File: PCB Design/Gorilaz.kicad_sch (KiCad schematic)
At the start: 47 parts, among them J1 Conn_01x13, J2 Conn_01x13, J3 Conn_01x13, J4 Conn_01x13, J5 HRO_TYPE-C-31-M-14, J6 Battery, J7 Conn_01x13, J8 Conn_01x13, J9 TC2030_SWD, Q2 2N7002, SW1 PWR, SW4 RST, U1 SRV05-4, U10 MAX17048, U3 BQ24075, U4 DW01A, U5 FS8205, U8 nRF52840_moko_mk08

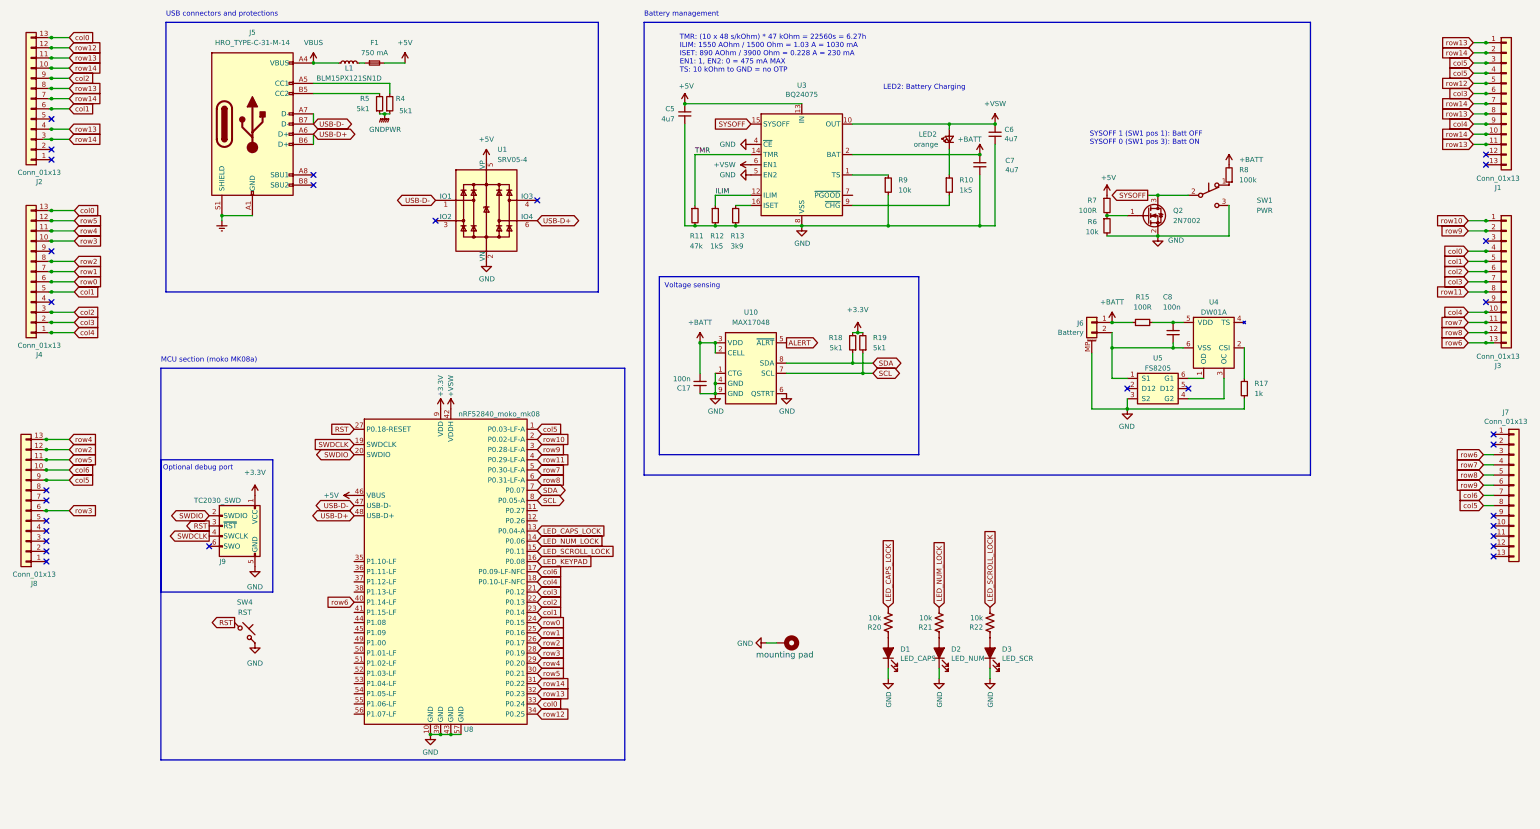
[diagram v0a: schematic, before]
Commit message: power managemnt rework
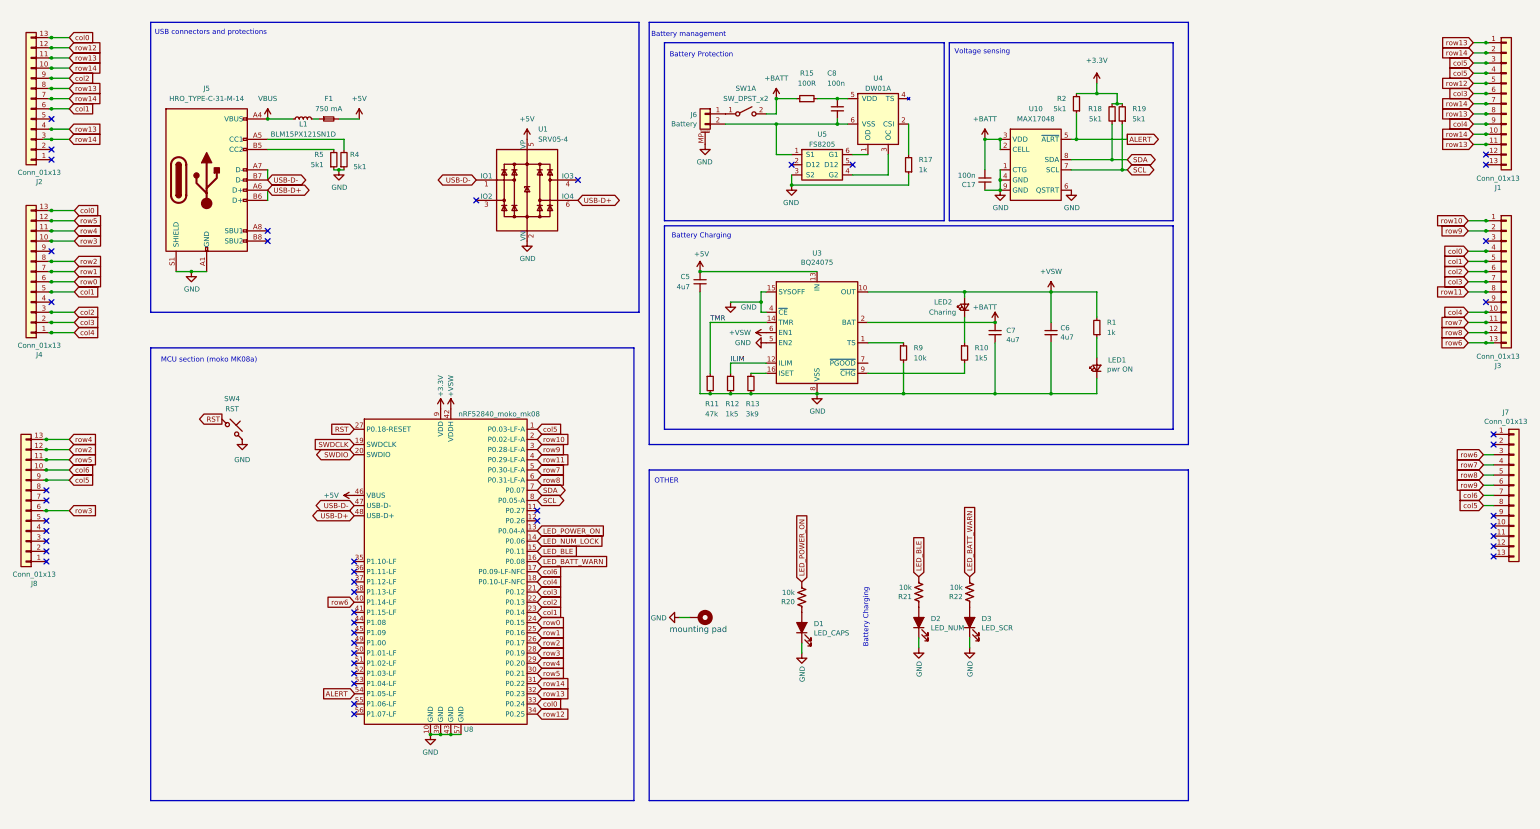
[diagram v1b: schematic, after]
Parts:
- removed J9: TC2030_SWD, Local:CON_TC2030_outlined, symbol PCM_marbastlib-various:TC2030_SWD
- removed Q2: 2N7002, Package_TO_SOT_SMD:SOT-23, symbol Transistor_FET:2N7002
- removed R6: 10k, Resistor_SMD:R_0402_1005Metric, symbol Device:R_Small
- removed R7: 100R, Resistor_SMD:R_0402_1005Metric, symbol Device:R_Small
- removed R8: 100k, Resistor_SMD:R_0402_1005Metric, symbol Device:R_Small
- removed SW1: PWR, Mastarlib:SW_MSK12C02-HB, symbol Switch:SW_Push_SPDT
- added LED1: pwr ON, LED_SMD:LED_0402_1005Metric, symbol Device:LED_Small
- added R1: 1k, Resistor_SMD:R_0402_1005Metric, symbol Device:R_Small
- added R2: 5k1, Resistor_SMD:R_0402_1005Metric, symbol Device:R_Small
- added SW1: SW_DPST_x2, symbol Switch:SW_DPST_x2
- LED2: value orange -> Charing
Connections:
- net GNDPWR is gone; now on net GND: R4.1, R5.1
- net SYSOFF is gone; now on net GND: U3.15 (SYSOFF)
- net +3.3V: now also R2.2
- net +BATT: now also SW1.2 (B); no longer J6.1 (Pin_1)
- net +VSW: now also R1.2
- net ALERT: now also R2.1
- net GND: now also LED1.1 (K)
- net LED_NUM_LOCK: no longer R21.2
- net LED_CAPS_LOCK renamed LED_POWER_ON
- net LED_KEYPAD renamed LED_BATT_WARN
- net LED_BATT_WARN: now also R22.2
- net LED_SCROLL_LOCK renamed LED_BLE
- net LED_BLE: now also R21.2; no longer R22.2
- new net: LED1.2 (A), R1.1
- new net: J6.1 (Pin_1), SW1.1 (A)
- no-connect marks 30 -> 45
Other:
- note added: "Battery Charging"
- note added: "Battery Protection"
- note added: "OTHER"
- note removed: "LED2: Battery Charging"
- note removed: "Optional debug port"
- note removed: "SYSOFF 1 (SW1 pos 1): Batt OFF SYSOFF 0 (SW1 pos 3): Batt ON"
- note removed: "TMR: (10 x 48 s/kOhm) * 47 kOhm = 22560s = 6.27h ILIM: 1550 AOhm / 1500 Ohm = 1.03 A = 1030 mA ISET: 890 AOhm / 3900 Ohm = 0.228 A = 230 mA EN1: 1, EN2: 0 = 475 mA MAX TS: 10 kOhm to GND = no OTP"
- moved on the sheet: C17, C5, C6, C7, C8, D1, D2, D3, F1, J5, J6, L1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

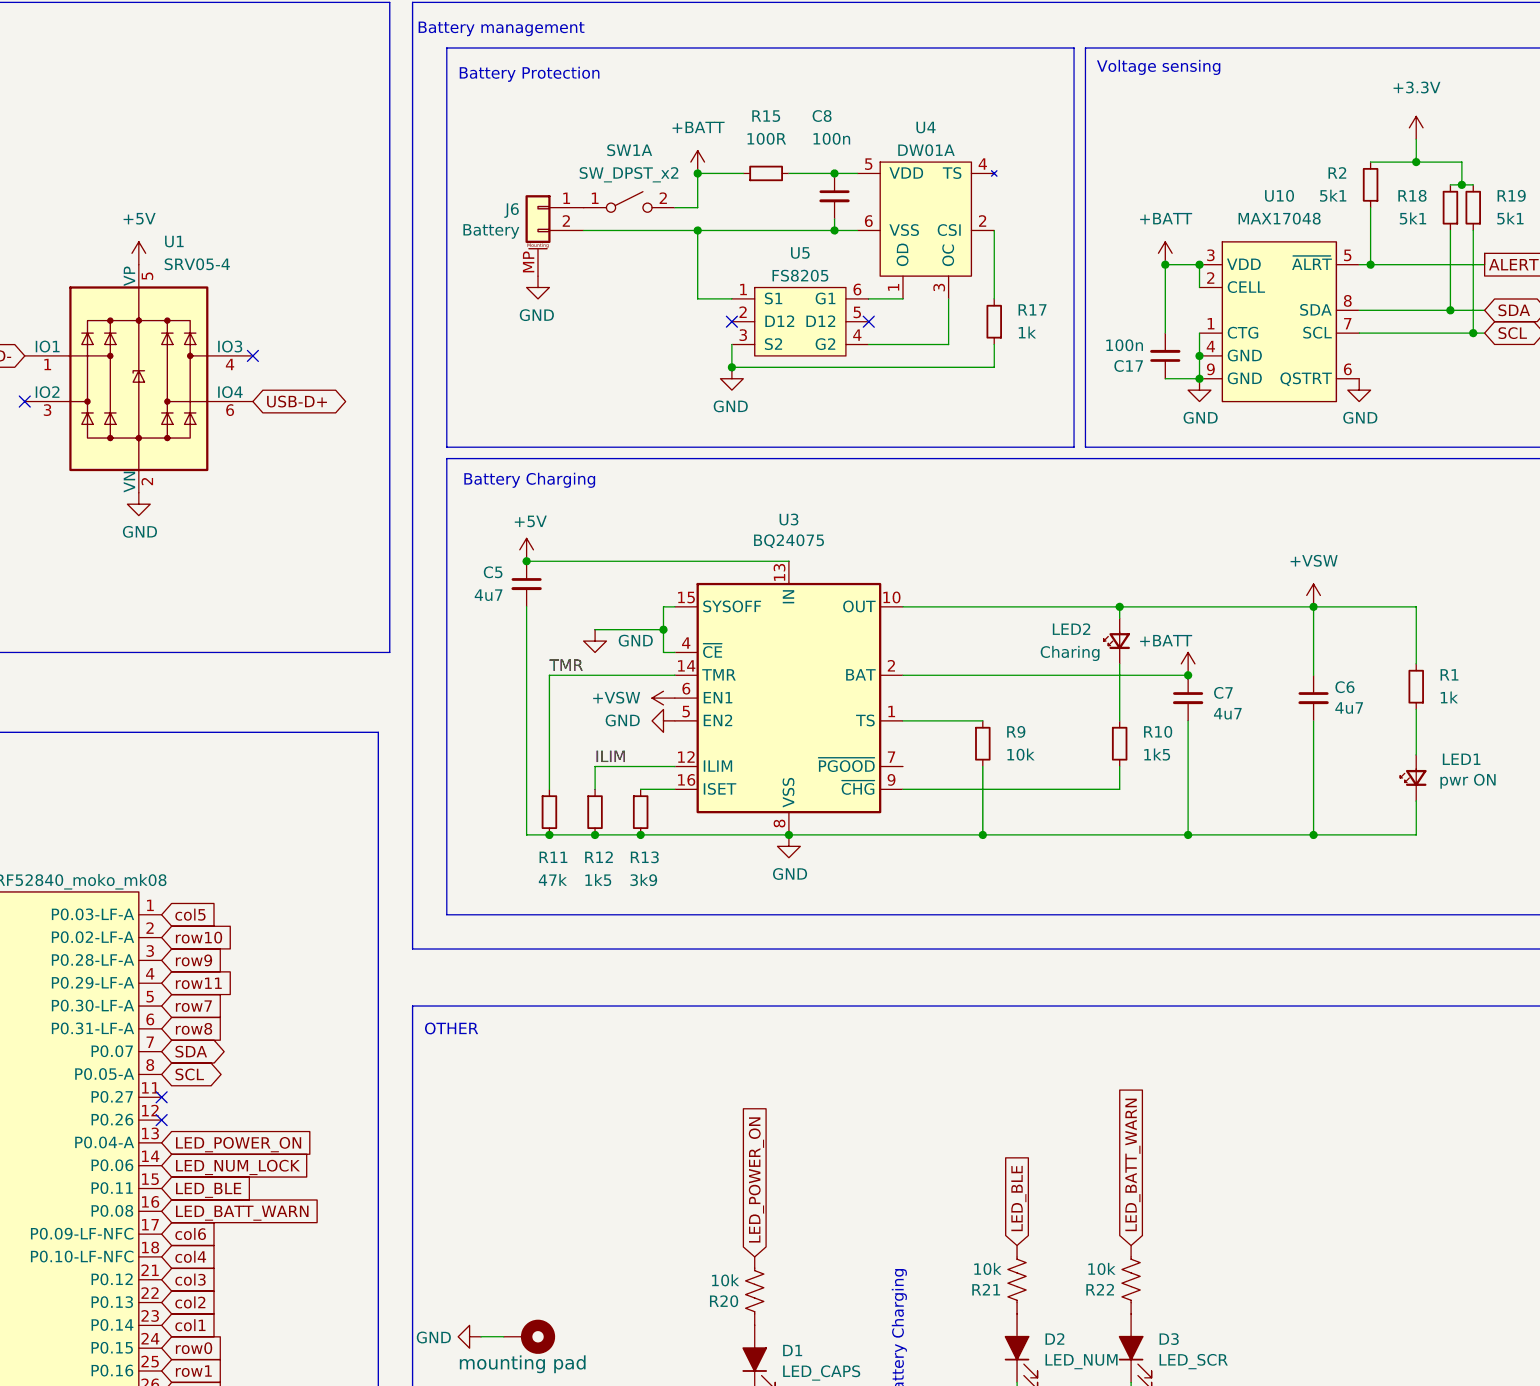
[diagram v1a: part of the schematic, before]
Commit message: big updates push
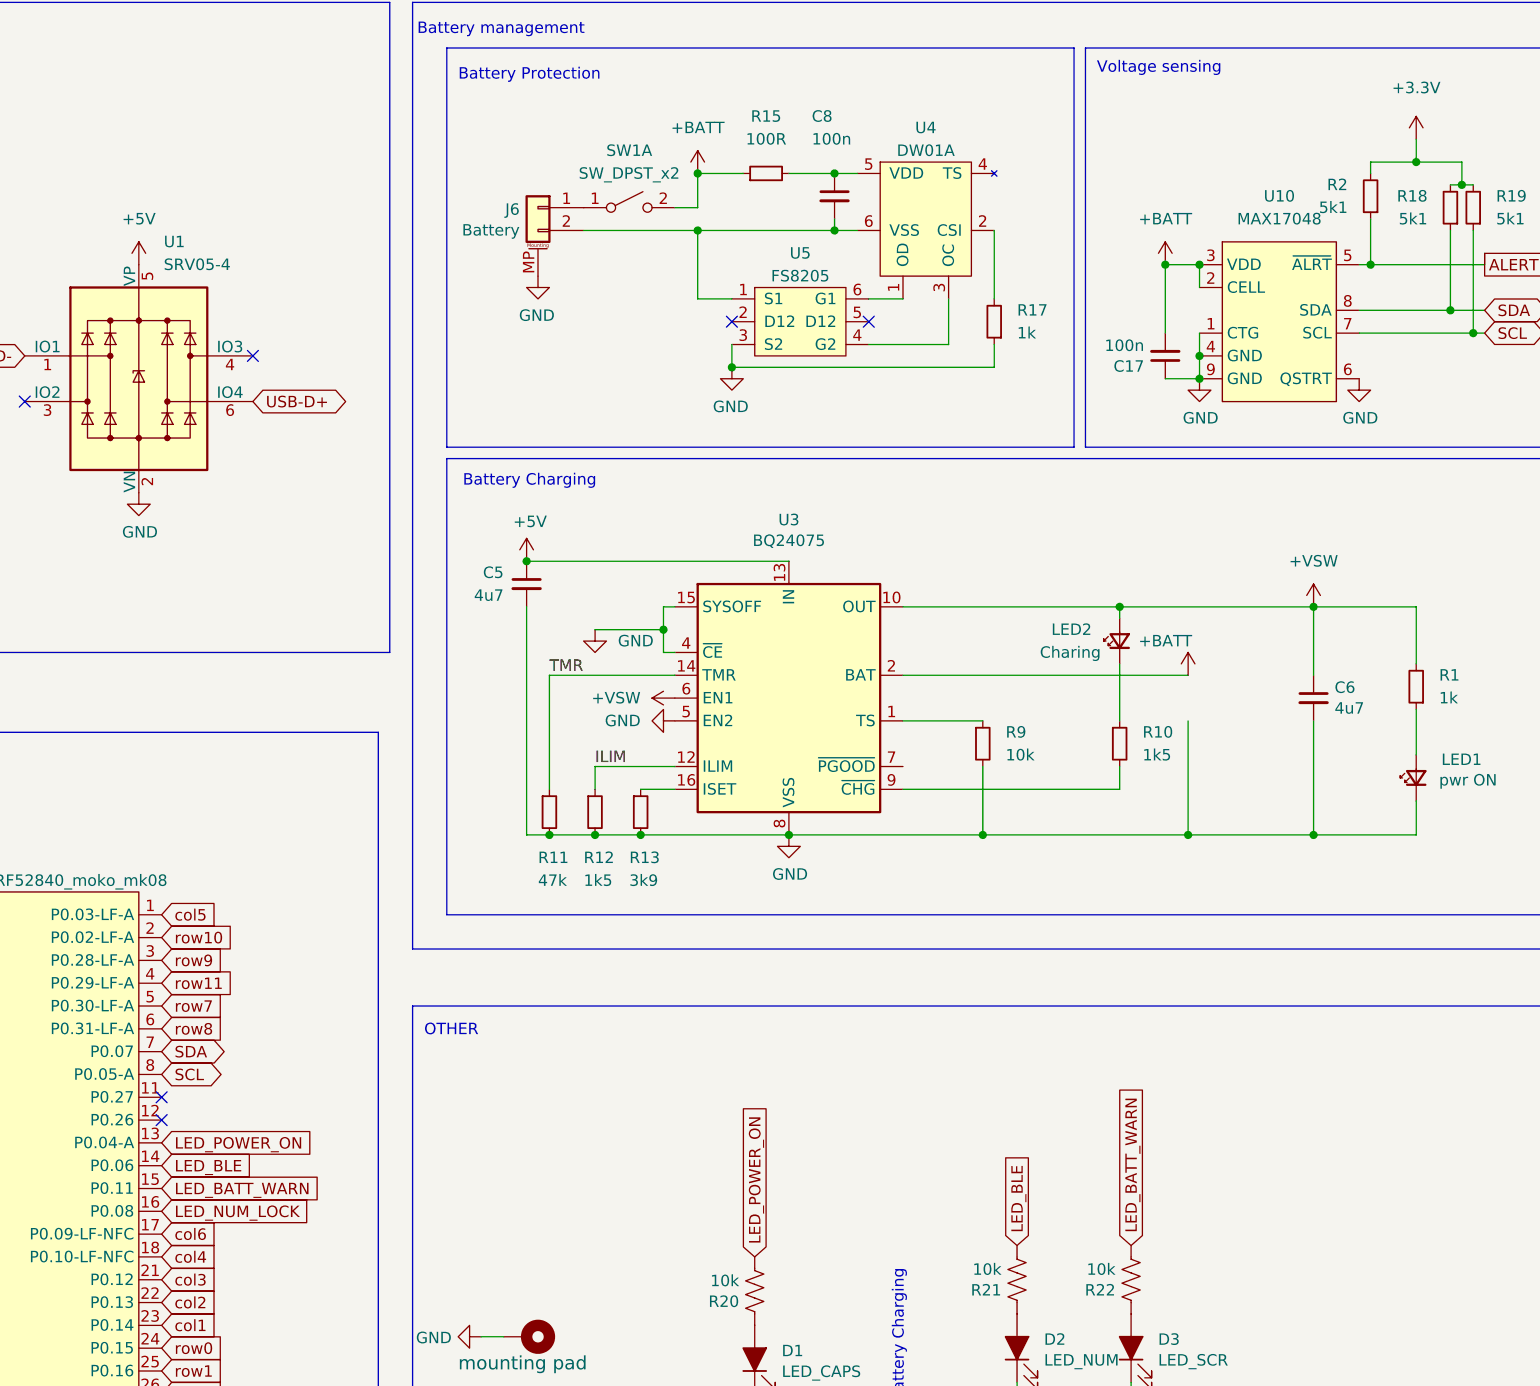
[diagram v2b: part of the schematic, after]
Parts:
- removed C7: 4u7, Capacitor_SMD:C_0402_1005Metric, symbol Device:C_Small
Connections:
- net LED_BATT_WARN: now also U8.15 (P0.11); no longer U8.16 (P0.08)
- net LED_BLE: now also U8.14 (P0.06); no longer U8.15 (P0.11)
- net LED_NUM_LOCK: now also U8.16 (P0.08); no longer U8.14 (P0.06)
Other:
- moved on the sheet: R2
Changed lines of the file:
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@@
 	)
 	(junction
-		(at 267.97 99.06)
-		(diameter 0.9144)
-		(color 0 0 0 0)
-	)
-	(junction
 		(at 132.08 201.93)
 		(diameter 0)
@@
 	(wire
 		(pts
-			(xy 293.37 41.91) (xy 298.45 41.91)
-		)
-		(stroke
-			(width 0)
-			(type default)
-		)
-	)
-	(wire
-		(pts
 			(xy 30.48 146.05) (xy 31.115 146.05)
 		)
@@
 	(wire
 		(pts
-			(xy 288.29 41.91) (xy 293.37 41.91)
-		)
-		(stroke
-			(width 0)
-			(type default)
-		)
-	)
-	(wire
-		(pts
 			(xy 390.525 39.37) (xy 391.16 39.37)
 		)
@@
 	(wire
 		(pts
+			(xy 293.37 41.91) (xy 298.45 41.91)
+		)
+		(stroke
+			(width 0)
+			(type default)
+		)
+	)
+	(wire
+		(pts
 			(xy 86.36 55.88) (xy 102.87 55.88)
 		)
@@
 	(wire
 		(pts
+			(xy 288.29 41.91) (xy 288.29 43.18)
+		)
+		(stroke
+			(width 0)
+			(type default)
+		)
+	)
+	(wire
+		(pts
 			(xy 31.75 50.8) (xy 32.385 50.8)
 		)
@@
 	(wire
 		(pts
-			(xy 288.29 46.99) (xy 288.29 53.34)
+			(xy 288.29 48.26) (xy 288.29 53.34)
 		)
 		(stroke
@@
 	(wire
 		(pts
+			(xy 288.29 41.91) (xy 293.37 41.91)
+		)
+		(stroke
+			(width 0)
+			(type default)
+		)
+	)
+	(wire
+		(pts
 			(xy 32.385 45.72) (xy 36.83 45.72)
 		)
@@
 		)
 	)
+	(global_label "LED_BATT_WARN"
+		(shape input)
+		(at 153.67 156.21 0)
+		(fields_autoplaced yes)
+		(effects
+			(font
+				(size 1.27 1.27)
+			)
+			(justify left)
+		)
+		(property "Intersheetrefs" "${INTERSHEET_REFS}"
+			(at 171.4718 156.21 0)
+			(effects
+				(font
+					(size 1.27 1.27)
+				)
+				(justify left)
+				(hide yes)
+			)
+		)
+	)
 	(global_label "col6"
 		(shape input)
@@
 		)
 	)
+	(global_label "LED_BLE"
+		(shape input)
+		(at 153.67 153.67 0)
+		(fields_autoplaced yes)
+		(effects
+			(font
+				(size 1.27 1.27)
+			)
+			(justify left)
+		)
+		(property "Intersheetrefs" "${INTERSHEET_REFS}"
+			(at 164.517 153.67 0)
+			(effects
+				(font
+					(size 1.27 1.27)
+				)
+				(justify left)
+				(hide yes)
+			)
+		)
+	)
 	(global_label "LED_BATT_WARN"
 		(shape input)
@@
 		)
 	)
-	(global_label "LED_BATT_WARN"
-		(shape input)
-		(at 153.67 158.75 0)
-		(fields_autoplaced yes)
-		(effects
-			(font
-				(size 1.27 1.27)
-			)
-			(justify left)
-		)
-		(property "Intersheetrefs" "${INTERSHEET_REFS}"
-			(at 171.4718 158.75 0)
-			(effects
-				(font
-					(size 1.27 1.27)
-				)
-				(justify left)
-				(hide yes)
-			)
-		)
-	)
 	(global_label "row4"
 		(shape input)
@@
 		)
 	)
-	(global_label "LED_BLE"
-		(shape input)
-		(at 153.67 156.21 0)
-		(fields_autoplaced yes)
-		(effects
-			(font
-				(size 1.27 1.27)
-			)
-			(justify left)
-		)
-		(property "Intersheetrefs" "${INTERSHEET_REFS}"
-			(at 164.517 156.21 0)
-			(effects
-				(font
-					(size 1.27 1.27)
-				)
-				(justify left)
-				(hide yes)
-			)
-		)
-	)
 	(global_label "col0"
 		(shape input)
@@
 		)
 	)
-	(global_label "LED_NUM_LOCK"
-		(shape input)
-		(at 153.67 153.67 0)
-		(fields_autoplaced yes)
-		(effects
-			(font
-				(size 1.27 1.27)
-			)
-			(justify left)
-		)
-		(property "Intersheetrefs" "${INTERSHEET_REFS}"
-			(at 171.0485 153.67 0)
-			(effects
-				(font
-					(size 1.27 1.27)
-				)
-				(justify left)
-				(hide yes)
-			)
-		)
-	)
 	(global_label "col6"
 		(shape input)
@@
 		)
 	)
+	(global_label "LED_NUM_LOCK"
+		(shape input)
+		(at 153.67 158.75 0)
+		(fields_autoplaced yes)
+		(effects
+			(font
+				(size 1.27 1.27)
+			)
+			(justify left)
+		)
+		(property "Intersheetrefs" "${INTERSHEET_REFS}"
+			(at 171.0485 158.75 0)
+			(effects
+				(font
+					(size 1.27 1.27)
+				)
+				(justify left)
+				(hide yes)
+			)
+		)
+	)
 	(global_label "LED_POWER_ON"
 		(shape input)
@@
 	)
 	(symbol
-		(lib_id "Device:C_Small")
-		(at 267.97 101.6 0)
-		(unit 1)
-		(exclude_from_sim no)
-		(in_bom yes)
-		(on_board yes)
-		(dnp no)
-		(property "Reference" "C7"
-			(at 270.764 101.0666 0)
-			(effects
-				(font
-					(size 1.27 1.27)
-				)
-				(justify left)
-			)
-		)
-		(property "Value" "4u7"
-			(at 270.764 103.378 0)
-			(effects
-				(font
-					(size 1.27 1.27)
-				)
-				(justify left)
-			)
-		)
-		(property "Footprint" "Capacitor_SMD:C_0402_1005Metric"
-			(at 267.97 101.6 0)
-			(effects
-				(font
-					(size 1.27 1.27)
-				)
-				(hide yes)
-			)
-		)
-		(property "Datasheet" "~"
-			(at 267.97 101.6 0)
-			(effects
-				(font
-					(size 1.27 1.27)
-				)
-				(hide yes)
-			)
-		)
-		(property "Description" ""
-			(at 267.97 101.6 0)
-			(effects
-				(font
-					(size 1.27 1.27)
-				)
-				(hide yes)
-			)
-		)
-		(property "LCSC" ""
-			(at 267.97 101.6 0)
-			(effects
-				(font
-					(size 1.27 1.27)
-				)
-				(hide yes)
-			)
-		)
-		(property "Notes" "X7R, 10%"
-			(at 267.97 101.6 0)
-			(effects
-				(font
-					(size 1.27 1.27)
-				)
-				(hide yes)
-			)
-		)
-		(pin "1"
-		)
-		(pin "2"
-		)
-		(instances
-			(project "Gorilaz"
-				(path "/46ef0abf-42df-44ff-8272-0b82956755c4"
-					(reference "C7")
-					(unit 1)
-				)
-			)
-		)
-	)
-	(symbol
 		(lib_id "Connector:USB_C_Receptacle_USB2.0")
 		(at 71.12 63.5 0)
@@
 	(symbol
 		(lib_id "Device:R_Small")
-		(at 288.29 44.45 180)
+		(at 288.29 45.72 180)
 		(unit 1)
 		(exclude_from_sim no)
@@
 		(dnp no)
 		(property "Reference" "R2"
-			(at 285.75 43.18 0)
+			(at 285.75 44.45 0)
 			(effects
 				(font
@@
 		)
 		(property "Value" "5k1"
-			(at 285.75 45.72 0)
+			(at 285.75 46.99 0)
 			(effects
 				(font
@@
 		)
 		(property "Footprint" "Resistor_SMD:R_0402_1005Metric"
-			(at 288.29 44.45 0)
+			(at 288.29 45.72 0)
 			(effects
 				(font
@@
 		)
 		(property "Datasheet" "~"
-			(at 288.29 44.45 0)
+			(at 288.29 45.72 0)
 			(effects
 				(font
@@
 		)
 		(property "Description" ""
-			(at 288.29 44.45 0)
+			(at 288.29 45.72 0)
 			(effects
 				(font
